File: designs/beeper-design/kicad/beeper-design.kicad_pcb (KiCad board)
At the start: 4 copper layers, 27.5 x 19 mm, 99 parts

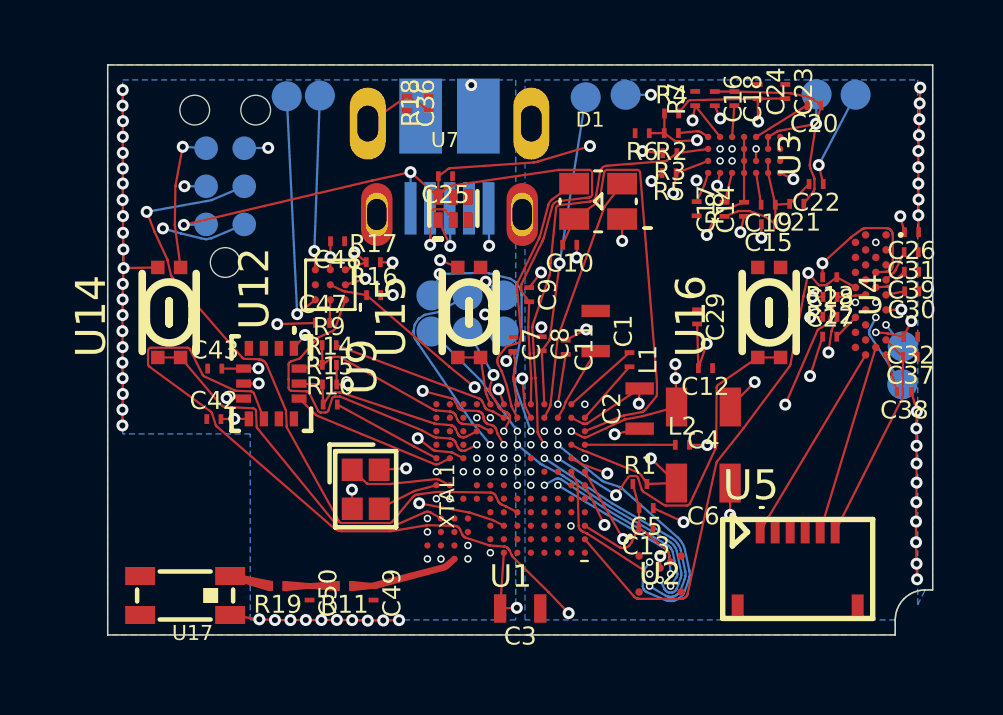
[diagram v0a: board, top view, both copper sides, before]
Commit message: new export
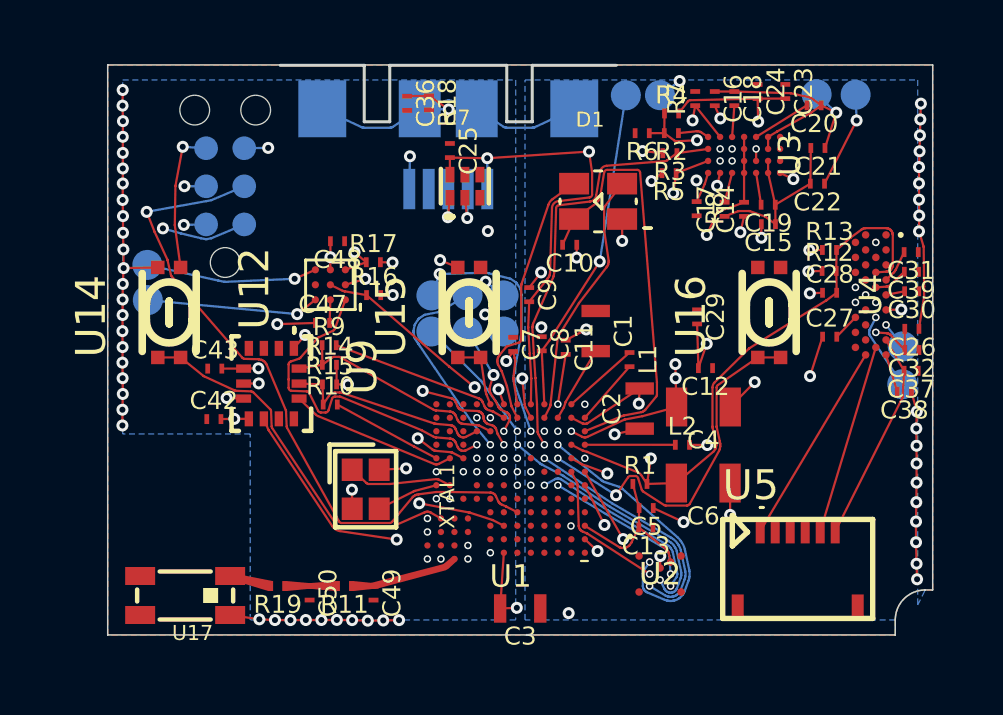
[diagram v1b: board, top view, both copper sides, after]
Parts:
- C10: footprint beeper-design:Pkg0201_18 -> beeper-design:Pkg0201_12
- C11: footprint beeper-design:Pkg0201_13 -> beeper-design:Pkg0201_5
- C12: footprint beeper-design:Pkg0201_31 -> beeper-design:Pkg0201_25
- C13: footprint beeper-design:Pkg0201_34 -> beeper-design:Pkg0201_28
- C14: footprint beeper-design:Pkg0201_2 -> beeper-design:Pkg0201
- C15: footprint beeper-design:Pkg0201_51 -> beeper-design:Pkg0201_50
- C16: footprint beeper-design:Pkg0201_12 -> beeper-design:Pkg0201_9
- C17: footprint beeper-design:Pkg0201_25 -> beeper-design:Pkg0201_22
- C18: footprint beeper-design:Pkg0201_37 -> beeper-design:Pkg0201_36
- C20: footprint beeper-design:Pkg0201_10 -> beeper-design:Pkg0201_7
- C21: footprint beeper-design:Pkg0201_23 -> beeper-design:Pkg0201_20
- C22: footprint beeper-design:Pkg0201_35 -> beeper-design:Pkg0201_33
- C24: footprint beeper-design:Pkg0201_7 -> beeper-design:Pkg0201_6
- C25: footprint beeper-design:Pkg0201_22 -> beeper-design:Pkg0201_18
- C26: footprint beeper-design:Pkg0201_42 -> beeper-design:Pkg0201_34
- C27: footprint beeper-design:Pkg0201_4 -> beeper-design:Pkg0201_53
- C28: footprint beeper-design:Pkg0201_47 -> beeper-design:Pkg0201_42
- C29: footprint beeper-design:Pkg0201_30 -> beeper-design:Pkg0201_24
- C30: footprint beeper-design:Pkg0201_16 -> beeper-design:Pkg0201_8
- C31: footprint beeper-design:Pkg0201_29 -> beeper-design:Pkg0201_21
- C32: footprint beeper-design:Pkg0201_17 -> beeper-design:Pkg0201_11
- C36: footprint beeper-design:Pkg0201_33 -> beeper-design:Pkg0201_30
- C37: footprint beeper-design:Pkg0201_45 -> beeper-design:Pkg0201_39
- C38: footprint beeper-design:Pkg0201_3 -> beeper-design:Pkg0201_51
- C39: footprint beeper-design:Pkg0201_1 -> beeper-design:Pkg0201_47
- C42: footprint beeper-design:Pkg0201_50 -> beeper-design:Pkg0201_43
- C43: footprint beeper-design:Pkg0201_9 -> beeper-design:Pkg0201_3
- C47: footprint beeper-design:Pkg0201_11 -> beeper-design:Pkg0201_4
- C48: footprint beeper-design:Pkg0201_24 -> beeper-design:Pkg0201_16
- C49: footprint beeper-design:Pkg0201_44 -> beeper-design:Pkg0201_37
- C5: footprint beeper-design:Pkg0201_6 -> beeper-design:Pkg0201_1
- C50: footprint beeper-design:Pkg0201_8 -> beeper-design:Pkg0201_2
- C7: footprint beeper-design:Pkg0201_32 -> beeper-design:Pkg0201_26
- C8: footprint beeper-design:Pkg0201_46 -> beeper-design:Pkg0201_41
- C9: footprint beeper-design:Pkg0201_5 -> beeper-design:Pkg0201_54
- J6: footprint beeper-design:AMPHENOL_10103594_0001LF -> beeper-design:GCT_USB3100_XX_X_REVB_1
- L1: footprint beeper-design:Pkg0201_40 -> beeper-design:Pkg0201_32
- L2: footprint beeper-design:Pkg0201_54 -> beeper-design:Pkg0201_46
- R1: footprint beeper-design:Pkg0201_27 -> beeper-design:Pkg0201_19
- R10: footprint beeper-design:Pkg0201_52 -> beeper-design:Pkg0201_44
- R11: footprint beeper-design:Pkg0201_53 -> beeper-design:Pkg0201_45
- R12, R13: footprint beeper-design:Pkg0201_36 -> beeper-design:Pkg0201_29
- R14, R15: footprint beeper-design:Pkg0201_20 -> beeper-design:Pkg0201_14
- R16, R17: footprint beeper-design:Pkg0201_39 -> beeper-design:Pkg0201_31
- R18: footprint beeper-design:Pkg0201_21 -> beeper-design:Pkg0201_17
- R19: footprint beeper-design:Pkg0201_19 -> beeper-design:Pkg0201_13
- R3: footprint beeper-design:Pkg0201_14 -> beeper-design:Pkg0201_10
- R4: footprint beeper-design:Pkg0201_41 -> beeper-design:Pkg0201_40
- R5: footprint beeper-design:Pkg0201 -> beeper-design:Pkg0201_52
- R6: footprint beeper-design:Pkg0201_28 -> beeper-design:Pkg0201_27
- R7: footprint beeper-design:Pkg0201_26 -> beeper-design:Pkg0201_23
- R9: footprint beeper-design:Pkg0201_43 -> beeper-design:Pkg0201_35
- moved TP1 8.22 mm to (127.1, 106.3)
- moved TP2 8.06 mm to (127.1, 105.2)
- moved C26 3.22 mm to (152.6, 107.3)
- moved C21 1.99 mm to (149.4, 101.3)
- moved TP11 1.34 mm to (143.0, 99.5)
- moved TP12 1.15 mm to (144.2, 99.5)
- moved R13 0.91 mm to (149.8, 104.7), turned to 90 degrees
- moved C25 0.87 mm to (137.2, 101.4), turned to 0 degrees
- moved R12 0.87 mm to (149.8, 105.4), turned to 90 degrees
- moved U7 0.84 mm to (137.7, 102.5)
- moved C28 0.80 mm to (149.8, 106.1)
- moved J6 0.49 mm to (137.1, 100.0)
- moved C37 0.46 mm to (152.5, 108.7)
- moved C32 0.44 mm to (152.6, 108.0)
- turned R18 to 0 degrees
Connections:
- net V14RF renamed V14
- net mcu_conn-uart_tx renamed mcu_mcu-uart_tx
- net mcu_dbg-m33_swdclk renamed mcu_mcu-dbg-m33_swdclk
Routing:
- net QVAR2: track 23.1 -> 6.47 mm, vias 1 -> 2
- net mcu_mcu-etm_data2: track 13.3 -> 7.71 mm
- net VBUS: track 40.2 -> 35.9 mm
- net SHIELD: track 7.91 -> 11.6 mm
- net VDD1P8P: track 22.8 -> 19.2 mm, vias 4 -> 1
- net VDD3P0: track 28.2 -> 25.1 mm, vias 5 -> 3
- net GND: track 51.2 -> 53.7 mm, vias 100 -> 101
- net codec-i2c-net_scl: track 18.0 -> 15.6 mm, vias 1 -> 3
- net OUT+: track 8.04 -> 5.77 mm
- net AC2: track 10.2 -> 8.80 mm
- net AC1: track 5.38 -> 6.53 mm
- net D-: track 18.3 -> 17.6 mm
- net codec-i2c-net_sda: track 12.7 -> 13.4 mm, vias 2 -> 3
- net VBAT: track 10.4 -> 10.9 mm
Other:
- outline, holes or cut-outs redrawn
